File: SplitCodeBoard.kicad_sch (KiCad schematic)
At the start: 3 parts

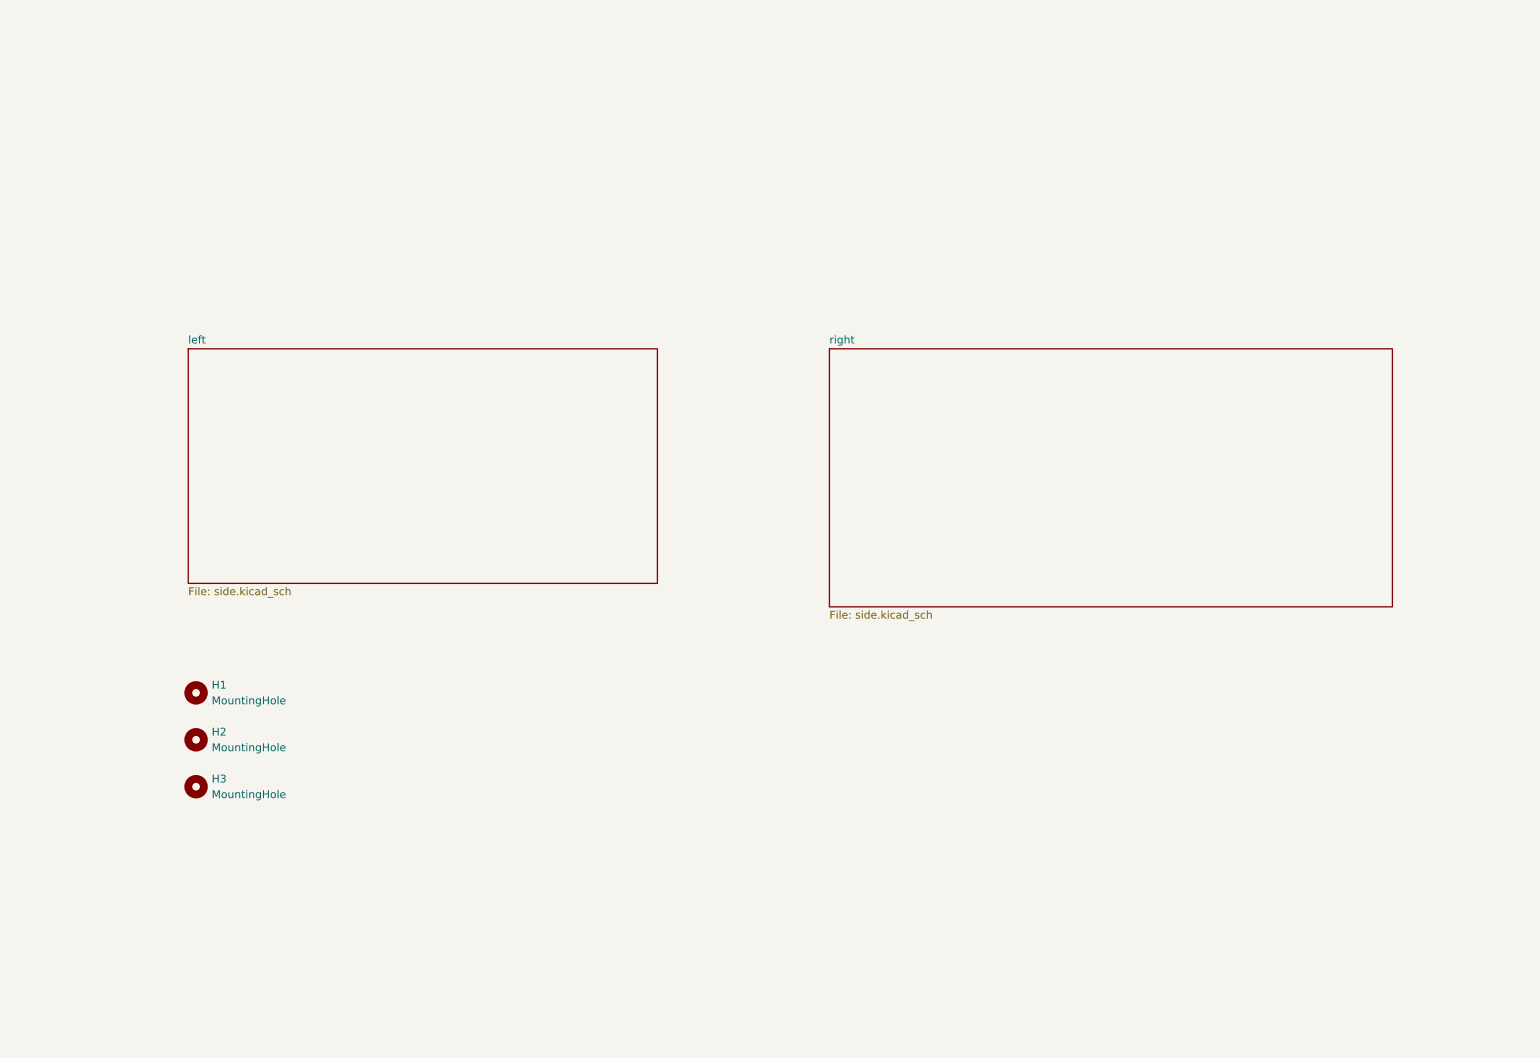
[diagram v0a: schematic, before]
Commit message: more stuff
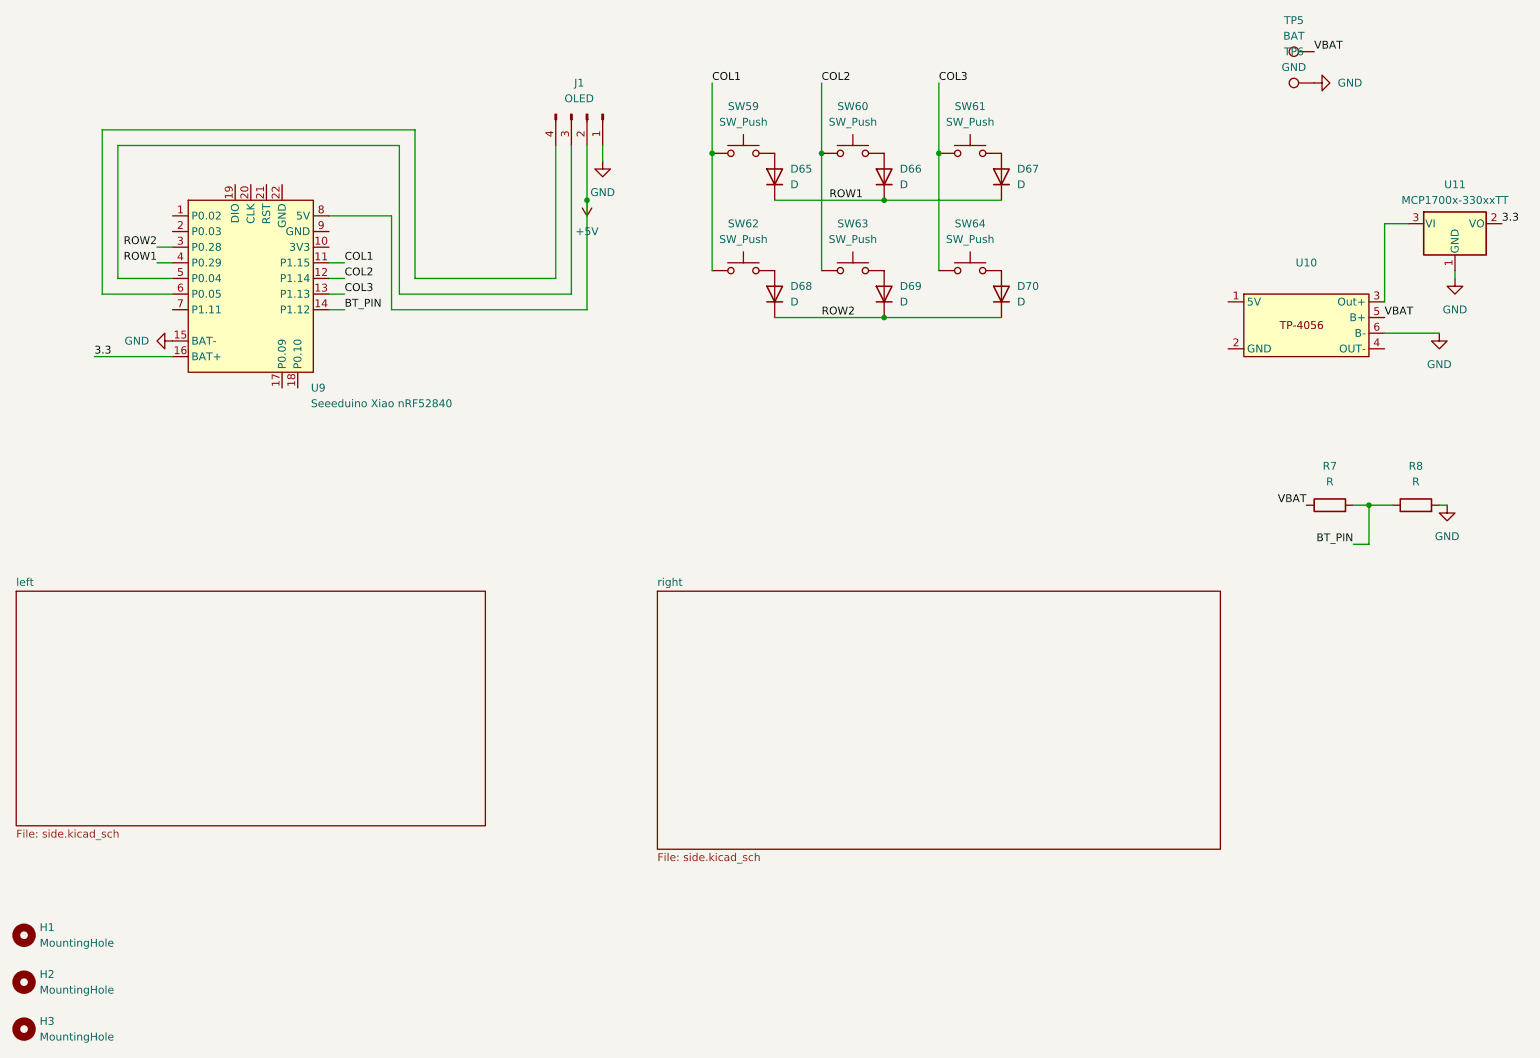
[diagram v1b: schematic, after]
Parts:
- added D65, D66, D67, D68, D69, D70: D, Diode_SMD:D_SOD-123, symbol Device:D
- added J1: OLED, KiCad-SSD1306-0.91-OLED-4pin-128x32:SSD1306-0.91-OLED-4pin-128x32, symbol Connector:Conn_01x04_Pin
- added R7, R8: R, Resistor_SMD:R_0201_0603Metric, symbol Device:R
- added SW59, SW60, SW61, SW62, SW63, SW64: SW_Push, PCM_marbastlib-choc:SW_choc_v1_HS_CPG135001S30_1u, symbol Switch:SW_Push
- added TP5: BAT, TestPoint:TestPoint_Pad_2.0x2.0mm, symbol Connector:TestPoint
- added TP6: GND, TestPoint:TestPoint_Pad_2.0x2.0mm, symbol Connector:TestPoint
- added U10: ~, TP4056:TP4056-18650, symbol TP4056:TP4056-18650
- added U11: MCP1700x-330xxTT, Package_TO_SOT_SMD:SOT-23, symbol Regulator_Linear:MCP1700x-330xxTT
- added U9: Seeeduino Xiao nRF52840, PCM_marbastlib-xp-promicroish:Xiao_nRF52840_ACH, symbol PCM_marbastlib-promicroish:Seeeduino_Xiao_nRF52840
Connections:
- new net: D66.2 (A), SW60.2
- new net: D65.2 (A), SW59.2
- new net: D70.2 (A), SW64.2
- new net: D69.2 (A), SW63.2
- new net: D67.2 (A), SW61.2
- new net: U10.3 (Out+), U11.3 (VI)
- new net: D68.2 (A), SW62.2
- new net: J1.3 (Pin_3), U9.5 (P0.04)
- new net: J1.4 (Pin_4), U9.6 (P0.05)
- new net +5V: J1.2 (Pin_2), U9.8 (5V)
- new net 3.3: U11.2 (VO), U9.16 (BAT+)
- new net BT_PIN: R7.2, R8.1, U9.14 (P1.12)
- new net COL1: SW59.1, SW62.1, U9.11 (P1.15)
- new net COL2: SW60.1, SW63.1, U9.12 (P1.14)
- new net COL3: SW61.1, SW64.1, U9.13 (P1.13)
- new net GND: J1.1 (Pin_1), R8.2, TP6.1, U10.6 (B-), U11.1 (GND), U9.15 (BAT-)
- new net ROW1: D65.1 (K), D66.1 (K), D67.1 (K), U9.4 (P0.29)
- new net ROW2: D68.1 (K), D69.1 (K), D70.1 (K), U9.3 (P0.28)
- new net VBAT: R7.1, TP5.1, U10.5 (B+)
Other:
- moved on the sheet: H1, H2, H3
